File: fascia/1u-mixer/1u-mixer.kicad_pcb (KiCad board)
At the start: 2 copper layers, 162.4 x 101.7 mm, 2 parts

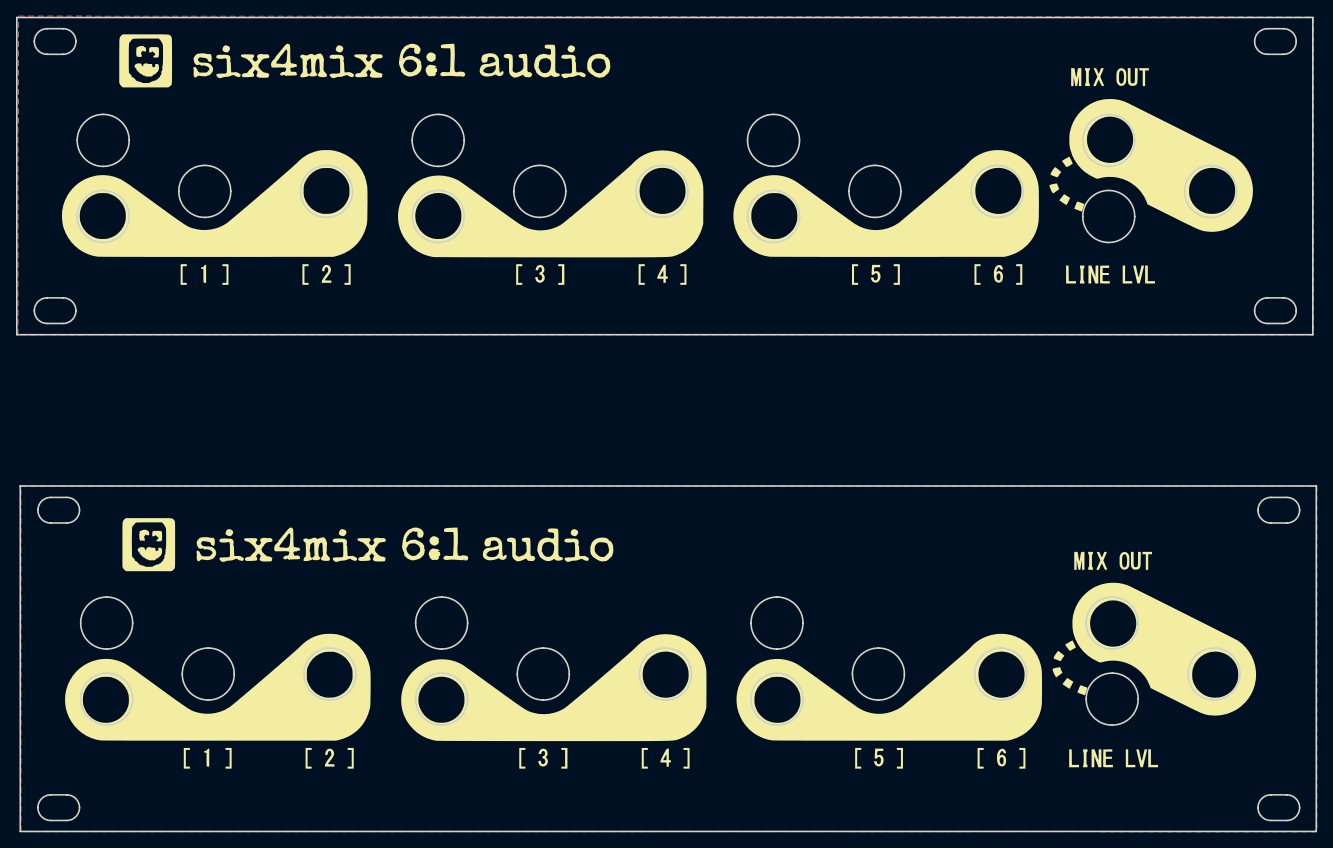
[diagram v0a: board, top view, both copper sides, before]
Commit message: Update 1u-mixer.kicad_pcb
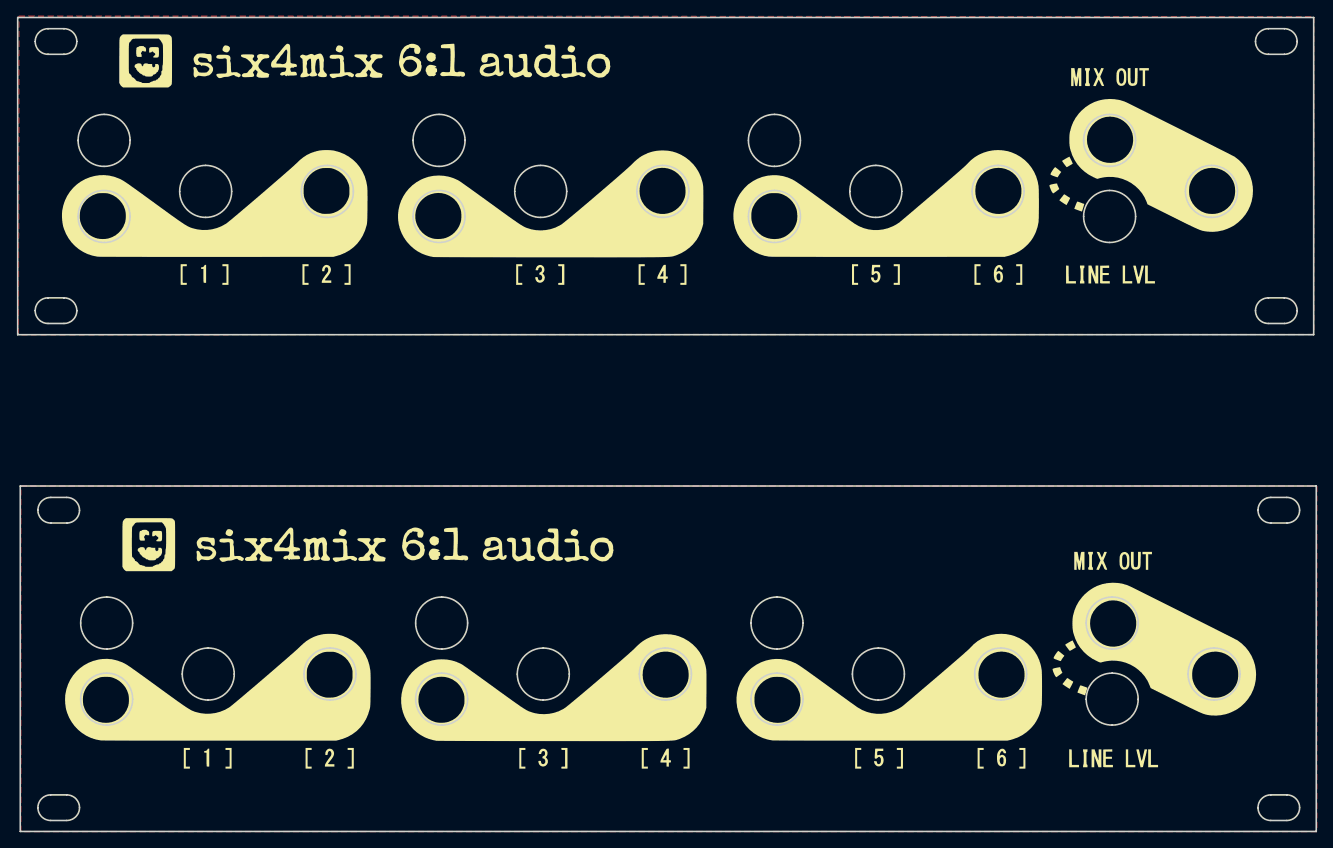
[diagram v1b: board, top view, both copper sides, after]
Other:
- board size 162.4 x 101.7 mm -> 162.3 x 101.7 mm
